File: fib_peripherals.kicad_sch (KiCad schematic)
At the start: 2 parts, among them J1 Conn_02x20_Odd_Even, J4 Conn_02x20_Odd_Even

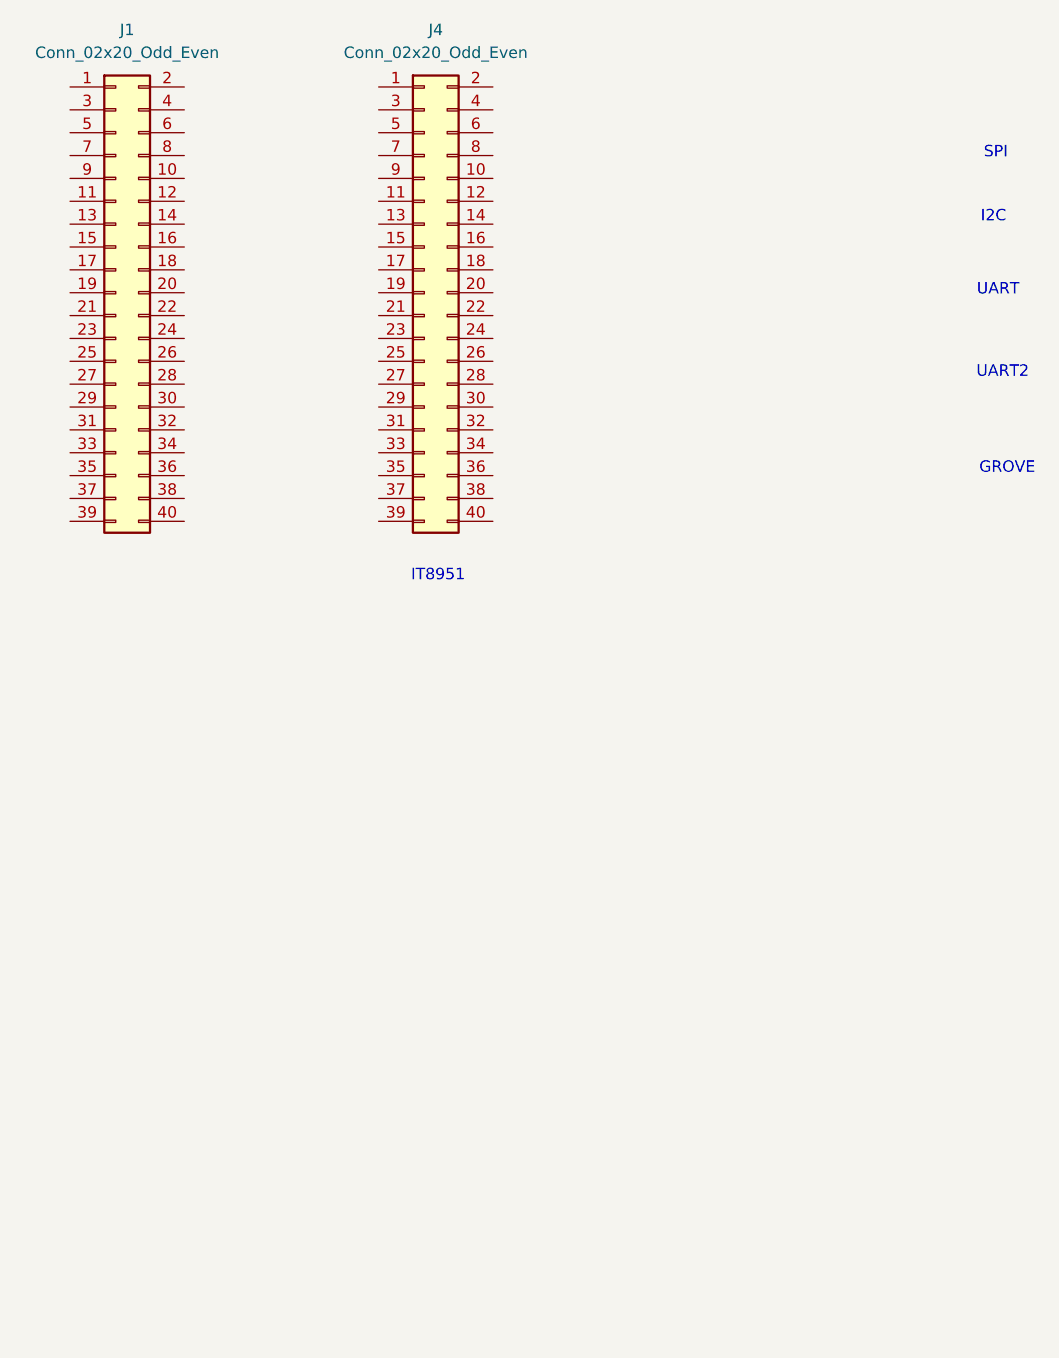
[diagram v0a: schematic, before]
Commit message: added symbol&footprint for orin/sodimm, added a bunch of specs and docs, partially implemented audio, full steam ahead
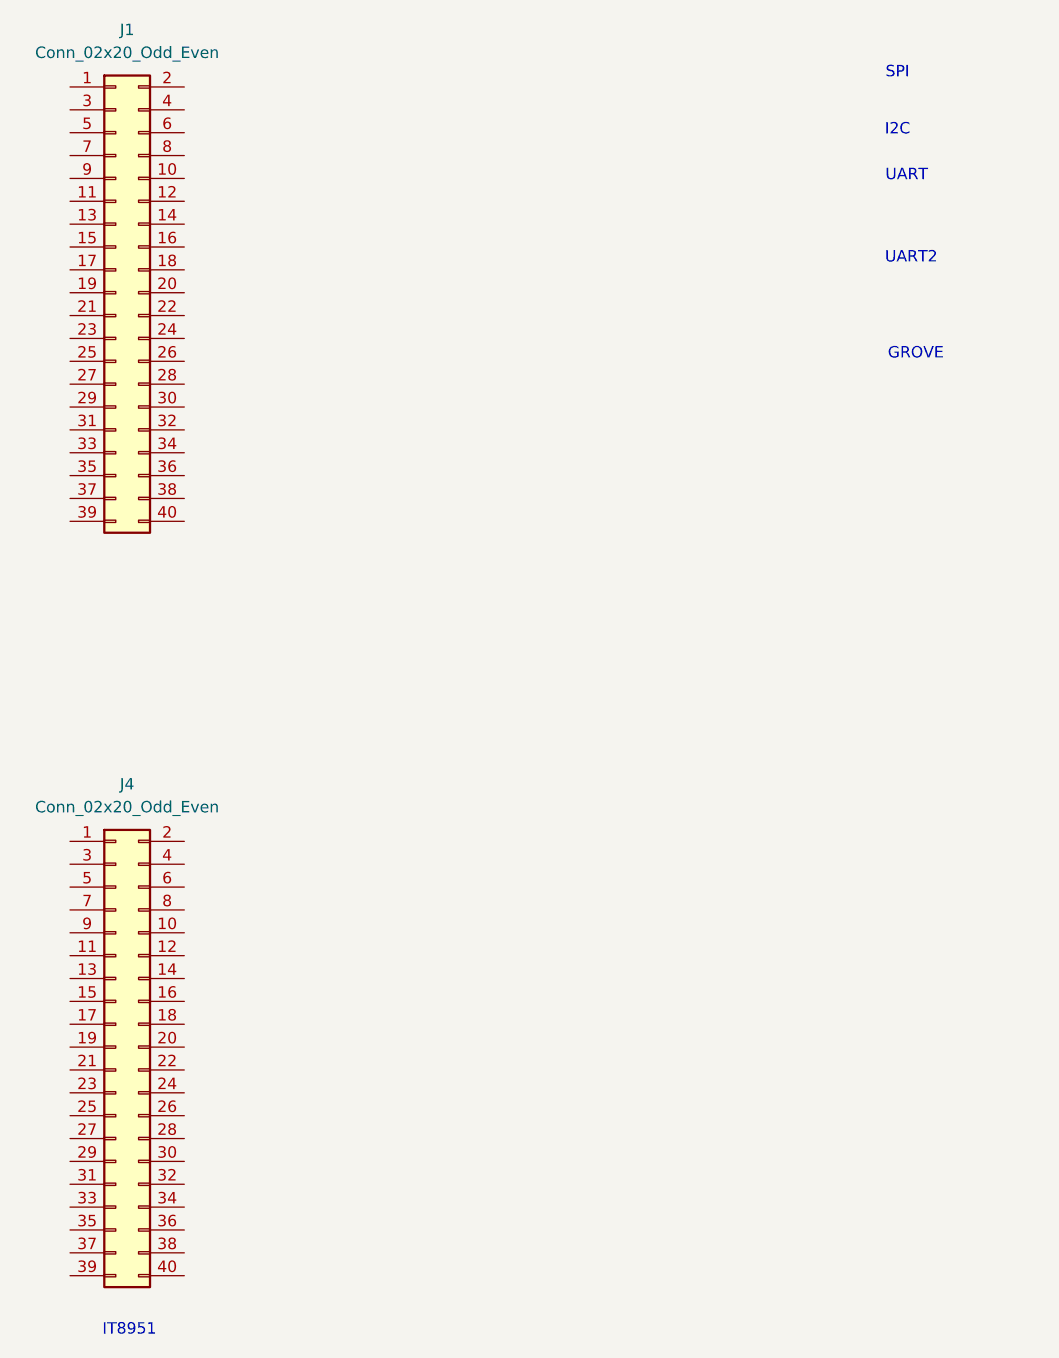
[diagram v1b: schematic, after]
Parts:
- J1, J4: footprint (none) -> Connector_PinHeader_2.54mm:PinHeader_2x20_P2.54mm_Vertical
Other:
- moved on the sheet: J4
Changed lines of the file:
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@@
 	(text "IT8951"
 		(exclude_from_sim no)
-		(at 77.724 88.646 0)
+		(at 43.434 172.466 0)
 		(effects
 			(font
@@
 	(text "I2C"
 		(exclude_from_sim no)
-		(at 139.446 48.768 0)
+		(at 128.778 39.116 0)
 		(effects
 			(font
@@
 	(text "UART"
 		(exclude_from_sim no)
-		(at 139.954 56.896 0)
+		(at 129.794 44.196 0)
 		(effects
 			(font
@@
 	(text "GROVE"
 		(exclude_from_sim no)
-		(at 140.97 76.708 0)
+		(at 130.81 64.008 0)
 		(effects
 			(font
@@
 	(text "UART2"
 		(exclude_from_sim no)
-		(at 140.462 66.04 0)
+		(at 130.302 53.34 0)
 		(effects
 			(font
@@
 	(text "SPI"
 		(exclude_from_sim no)
-		(at 139.7 41.656 0)
+		(at 128.778 32.766 0)
 		(effects
 			(font
@@
 			)
 		)
-		(property "Footprint" ""
+		(property "Footprint" "Connector_PinHeader_2.54mm:PinHeader_2x20_P2.54mm_Vertical"
 			(at 41.91 57.15 0)
 			(effects
@@
 	(symbol
 		(lib_id "Connector_Generic:Conn_02x20_Odd_Even")
-		(at 76.2 57.15 0)
+		(at 41.91 140.97 0)
 		(unit 1)
 		(exclude_from_sim no)
@@
 		(fields_autoplaced yes)
 		(property "Reference" "J4"
-			(at 77.47 27.94 0)
+			(at 43.18 111.76 0)
 			(effects
 				(font
@@
 		)
 		(property "Value" "Conn_02x20_Odd_Even"
-			(at 77.47 30.48 0)
-			(effects
-				(font
-					(size 1.27 1.27)
-				)
-			)
-		)
-		(property "Footprint" ""
-			(at 76.2 57.15 0)
+			(at 43.18 114.3 0)
+			(effects
+				(font
+					(size 1.27 1.27)
+				)
+			)
+		)
+		(property "Footprint" "Connector_PinHeader_2.54mm:PinHeader_2x20_P2.54mm_Vertical"
+			(at 41.91 140.97 0)
 			(effects
 				(font
@@
 		)
 		(property "Datasheet" "~"
-			(at 76.2 57.15 0)
+			(at 41.91 140.97 0)
 			(effects
 				(font
@@
 		)
 		(property "Description" "Generic connector, double row, 02x20, odd/even pin numbering scheme (row 1 odd numbers, row 2 even numbers), script generated (kicad-library-utils/schlib/autogen/connector/)"
-			(at 76.2 57.15 0)
-			(effects
-				(font
+			(at 41.91 140.97 0)
+			(effects
+				(font
